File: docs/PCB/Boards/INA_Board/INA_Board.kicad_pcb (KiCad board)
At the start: 2 copper layers, 64.2 x 35.6 mm, 21 parts, among them J1 COM, J2 INA, Q1 AO3407A, SW1 SW_DIP_x02, U1 INA226AIDGST, U2 SIP32431DR3-T1GE3

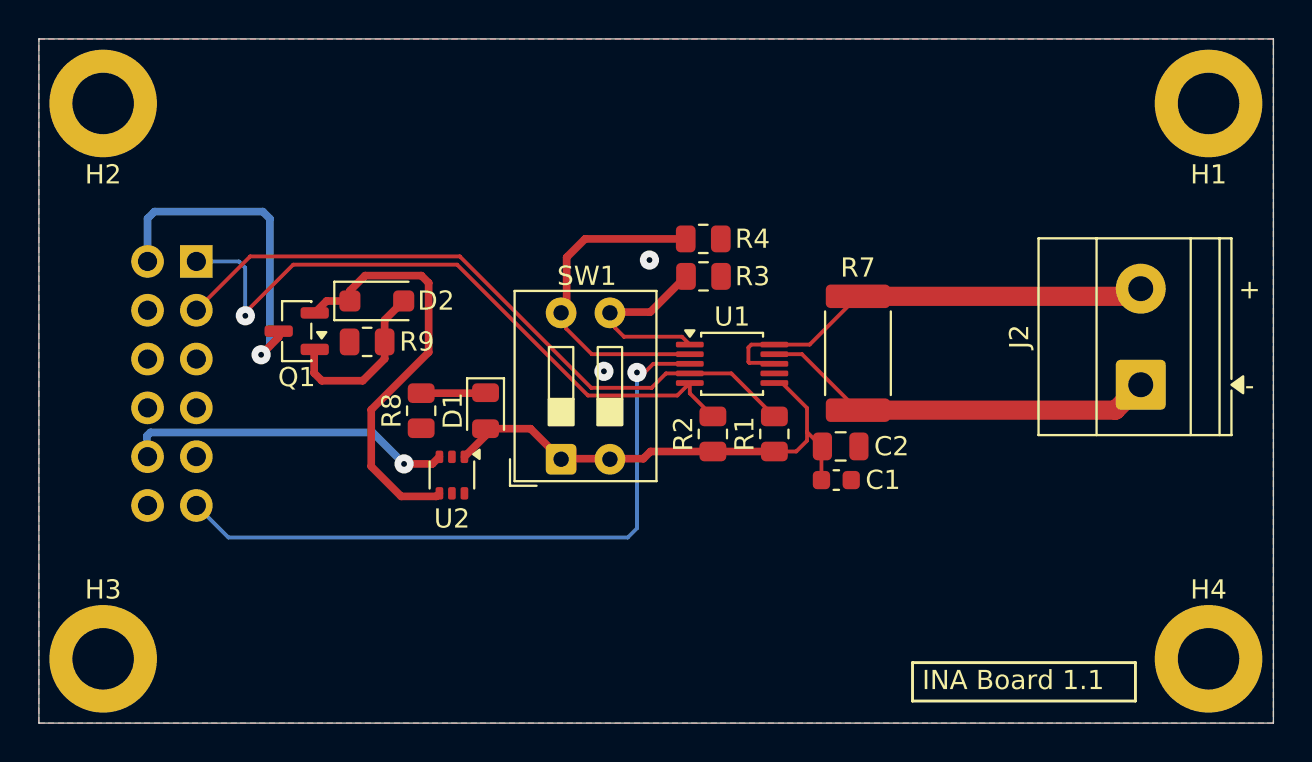
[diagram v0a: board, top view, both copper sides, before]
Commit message: Boards modified.
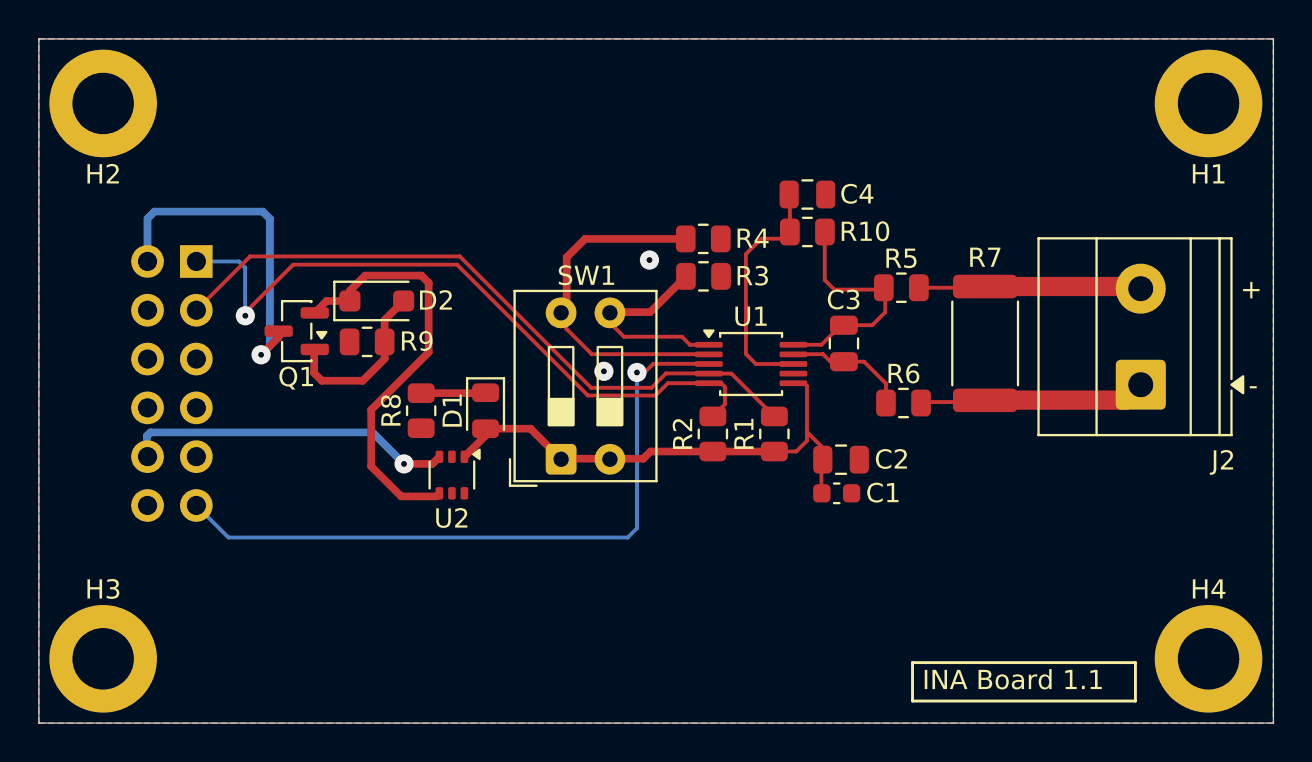
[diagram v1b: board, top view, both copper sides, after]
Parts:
- added C3: 100nF, Capacitor_SMD:C_0805_2012Metric, F.Cu at (157.5, 81.5)
- added C4: 100nF, Capacitor_SMD:C_0805_2012Metric, F.Cu at (155.6, 73.8)
- added R10: 10R, Resistor_SMD:R_0805_2012Metric, F.Cu at (155.6, 75.8)
- added R5: 10R, Resistor_SMD:R_0805_2012Metric, F.Cu at (160.5, 78.7)
- added R6: 10R, Resistor_SMD:R_0805_2012Metric, F.Cu at (160.6, 84.7)
- moved R7 6.64 mm to (164.8, 81.5)
- moved U1 0.99 mm to (152.7, 82.6)
- moved C1 0.69 mm to (157.1, 89.3)
- moved C2 0.69 mm to (157.3, 87.6)
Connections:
- U1 pad 10: INA+ -> Net-(U1-Vin+)
- U1 pad 8: INA+ -> Net-(U1-Vbus)
- U1 pad 9: INA- -> Net-(U1-Vin-)
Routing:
- net Net-(U1-Vin+): track 0.00 -> 13.0 mm
- net Net-(U1-Vbus): track 0.00 -> 12.5 mm
- net INA+: track 24.4 -> 12.7 mm
- net INA-: track 20.9 -> 13.4 mm
- net Net-(U1-Vin-): track 0.00 -> 6.20 mm
- net I2C0_SCL: track 34.8 -> 36.3 mm
- net Net-(U1-A0): track 17.3 -> 18.3 mm
- net Alert: track 34.9 -> 35.9 mm
- net Net-(U1-A1): track 9.65 -> 10.6 mm
